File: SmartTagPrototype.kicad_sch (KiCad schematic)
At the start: 56 parts, among them IC1 NRF52810-QFAA-R7, IC3 AEM30940-QFN, J1 Nordic output antenna, J10 SWD, J11 Port 9 -10, J12 Port 0 - 5, J2 Capacitor Voltage, J3 UART, J4 Port 11 - 18, J6 Port 22- 24, J7 Additional AC pins, J8 Conn_Coaxial, J9 AC pins (generator/antenna), X1 32MHz

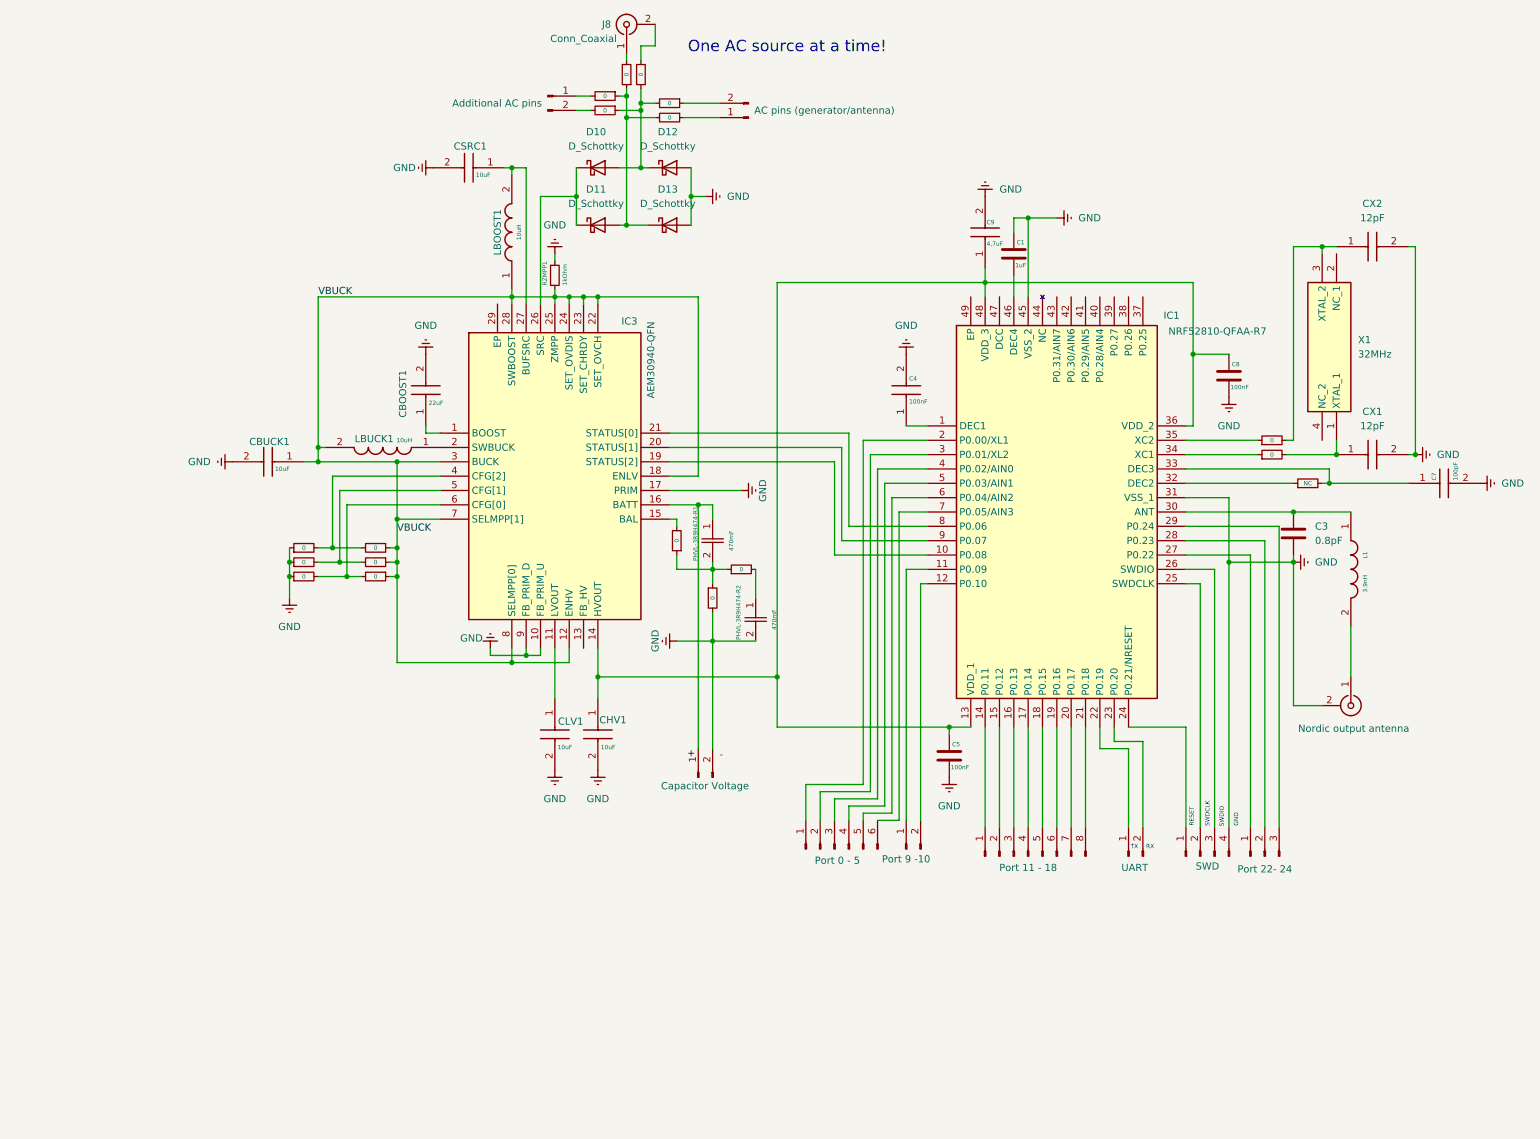
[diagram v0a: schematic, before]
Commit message: push abominacji czytaj dodany footprint i symbol zlacza testowego (niech Bog ma mnie w opiece)
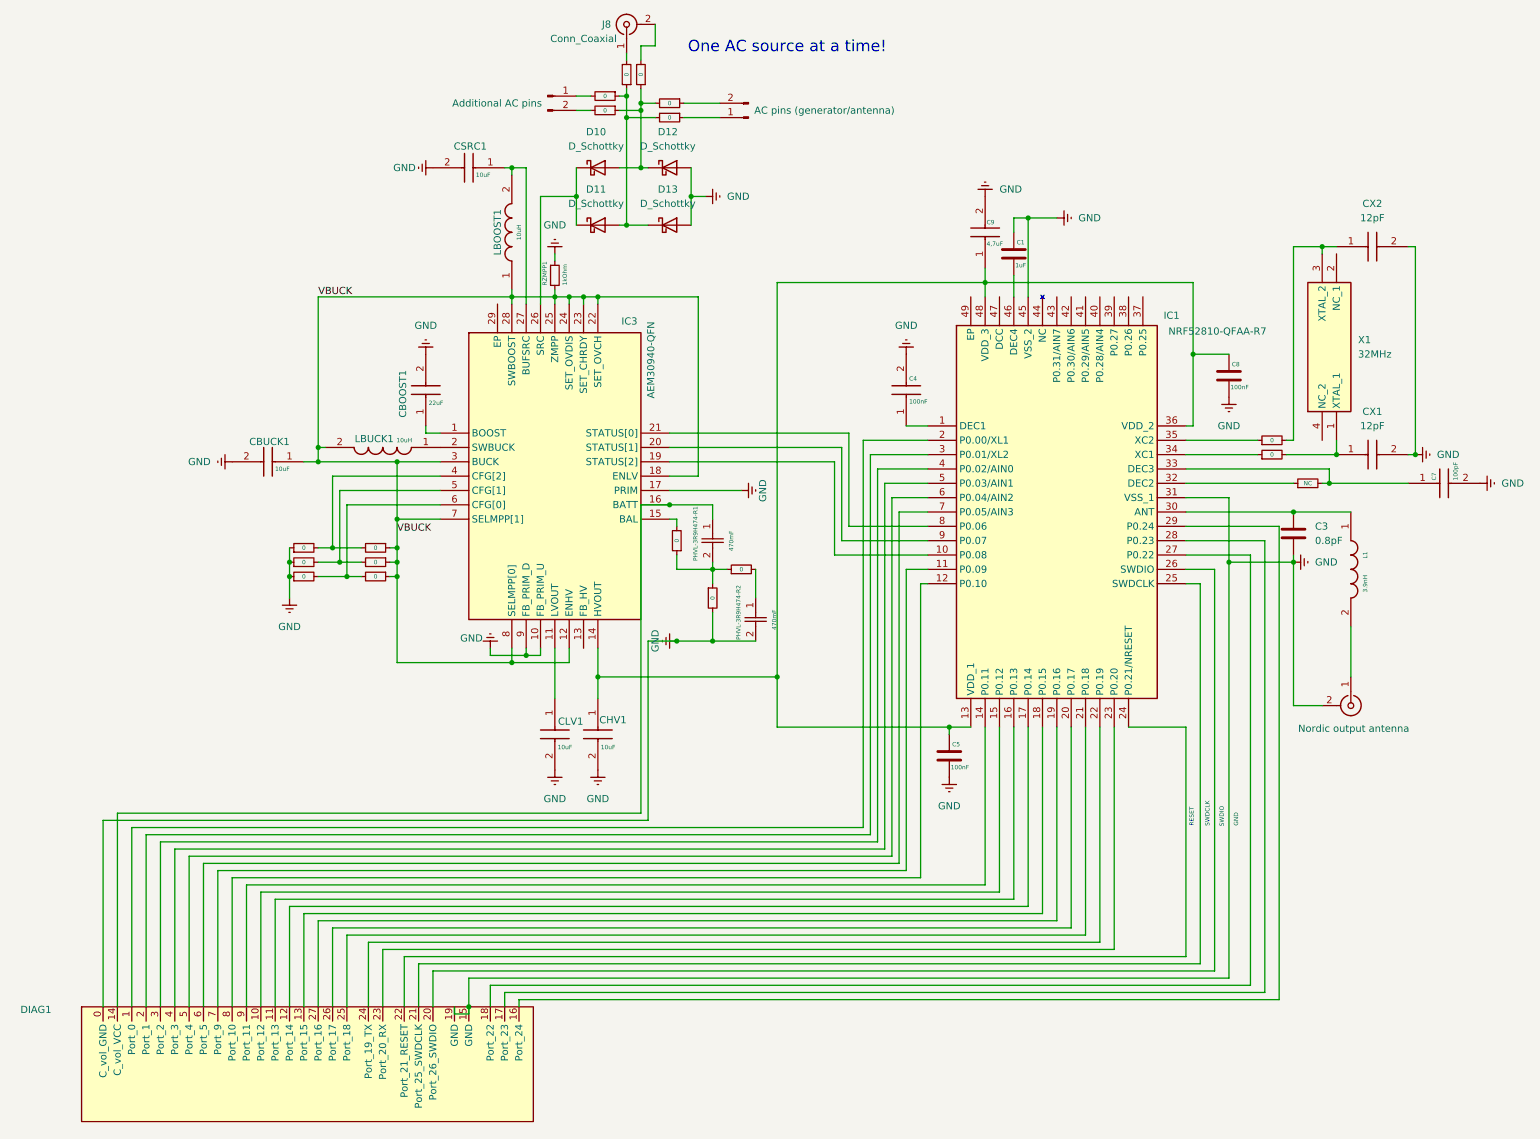
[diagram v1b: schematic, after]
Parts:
- removed J10: SWD, symbol Connector:Conn_01x04_Pin
- removed J11: Port 9 -10, symbol Connector:Conn_01x02_Pin
- removed J12: Port 0 - 5, symbol Connector:Conn_01x06_Pin
- removed J2: Capacitor Voltage, symbol Connector:Conn_01x02_Pin
- removed J3: UART, symbol Connector:Conn_01x02_Pin
- removed J4: Port 11 - 18, symbol Connector:Conn_01x08_Pin
- removed J6: Port 22- 24, symbol Connector:Conn_01x03_Pin
- added DIAG1: ~, Library:DIAG, symbol Library:Diag
- J7, J9: footprint (none) -> Connector_PinHeader_2.54mm:PinHeader_1x02_P2.54mm_Vertical
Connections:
- net GND: now also DIAG1.0 (C_vol_GND), DIAG1.15 (GND), DIAG1.19 (GND)
- net at IC1.22 (P0.19): now also DIAG1.24 (Port_19_TX)
- net at IC1.23 (P0.20): now also DIAG1.23 (Port_20_RX)
- net at IC1.11 (P0.09): now also DIAG1.7 (Port_9)
- net at IC1.12 (P0.10): now also DIAG1.8 (Port_10)
- net at IC1.2 (P0.00/XL1): now also DIAG1.1 (Port_0)
- net at IC1.3 (P0.01/XL2): now also DIAG1.2 (Port_1)
- net at IC1.4 (P0.02/AIN0): now also DIAG1.3 (Port_2)
- net at IC1.5 (P0.03/AIN1): now also DIAG1.4 (Port_3)
- net at IC1.6 (P0.04/AIN2): now also DIAG1.5 (Port_4)
- net at IC1.7 (P0.05/AIN3): now also DIAG1.6 (Port_5)
- net at IC3.16 (BATT), PHVL-3R9H474-R1.1: now also DIAG1.14 (C_vol_VCC)
- net at IC1.14 (P0.11): now also DIAG1.9 (Port_11)
- net at IC1.15 (P0.12): now also DIAG1.10 (Port_12)
- net at IC1.16 (P0.13): now also DIAG1.11 (Port_13)
- net at IC1.17 (P0.14): now also DIAG1.12 (Port_14)
- net at IC1.18 (P0.15): now also DIAG1.13 (Port_15)
- net at IC1.19 (P0.16): now also DIAG1.27 (Port_16)
- net at IC1.20 (P0.17): now also DIAG1.26 (Port_17)
- net at IC1.21 (P0.18): now also DIAG1.25 (Port_18)
- net at IC1.24 (P0.21/NRESET): now also DIAG1.22 (Port_21_RESET)
- net at IC1.25 (SWDCLK): now also DIAG1.21 (Port_25_SWDCLK)
- net at IC1.26 (SWDIO): now also DIAG1.20 (Port_26_SWDIO)
- net at IC1.27 (P0.22): now also DIAG1.18 (Port_22)
- net at IC1.28 (P0.23): now also DIAG1.17 (Port_23)
- net at IC1.29 (P0.24): now also DIAG1.16 (Port_24)
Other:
- note removed: "+"
- note removed: "-"
- note removed: "RX"
- note removed: "TX"
